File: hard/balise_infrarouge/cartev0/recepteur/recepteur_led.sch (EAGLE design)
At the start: 112 parts, among them IC2 7805DT, IC3 4051D, IC4 4051D, IC5 AT90CAN128A, J1 CAN, Q2 16M, X4 UART, X5 ISP

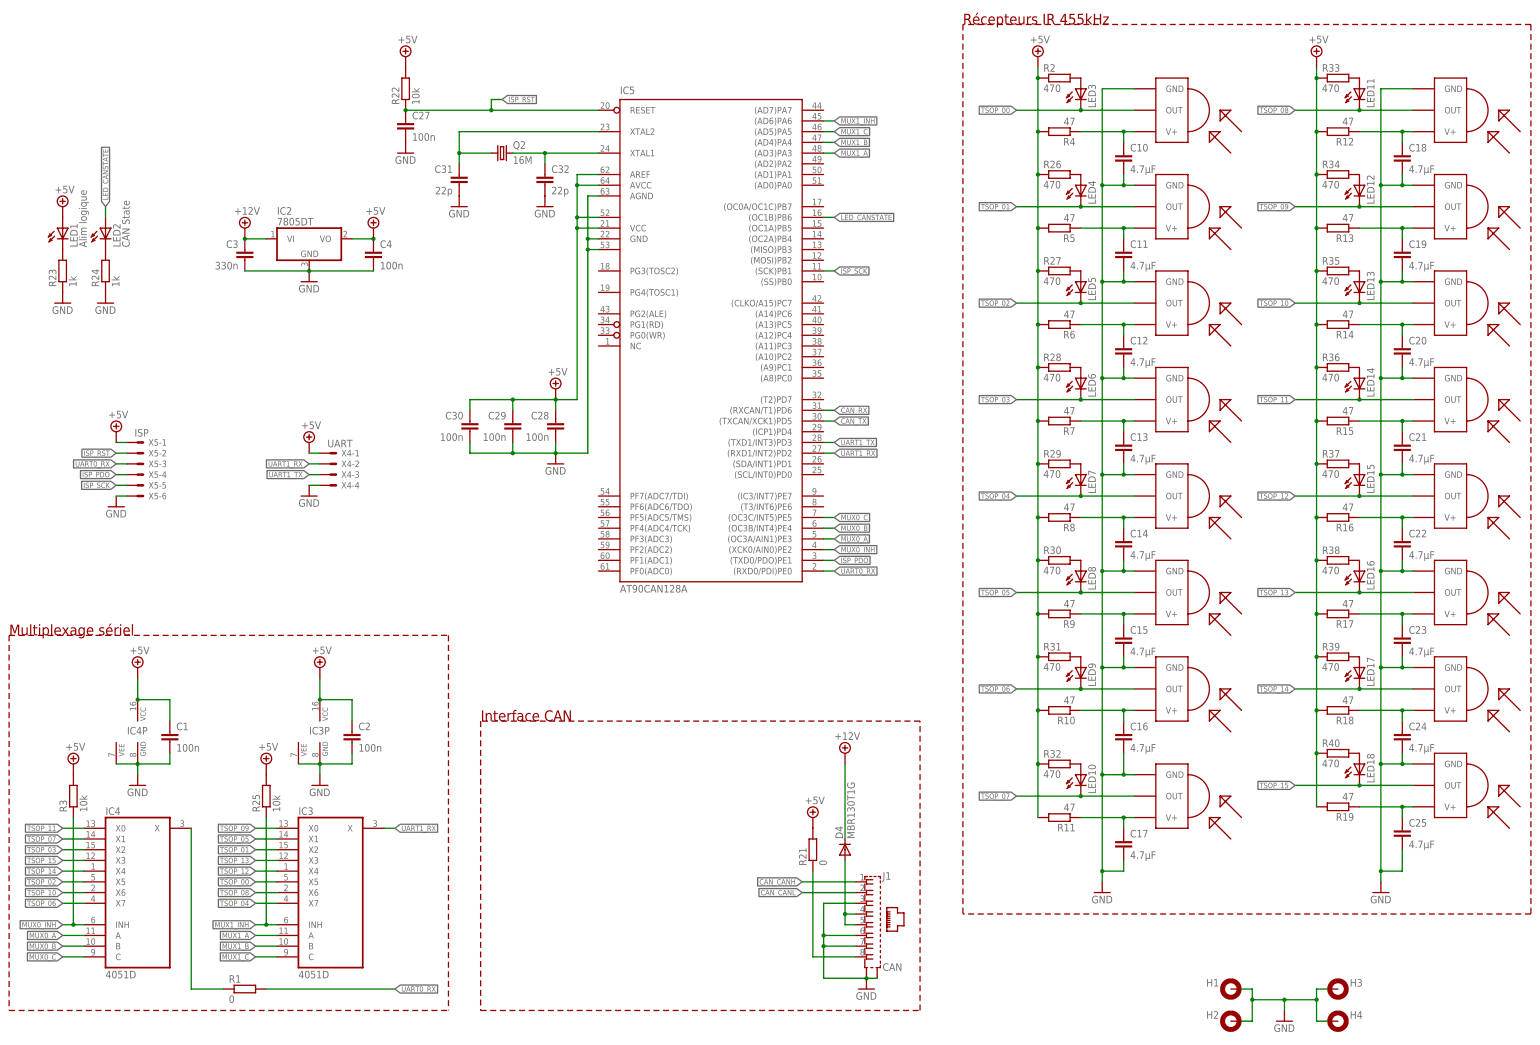
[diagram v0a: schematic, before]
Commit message: maj emetteur + fini recepteur part 1
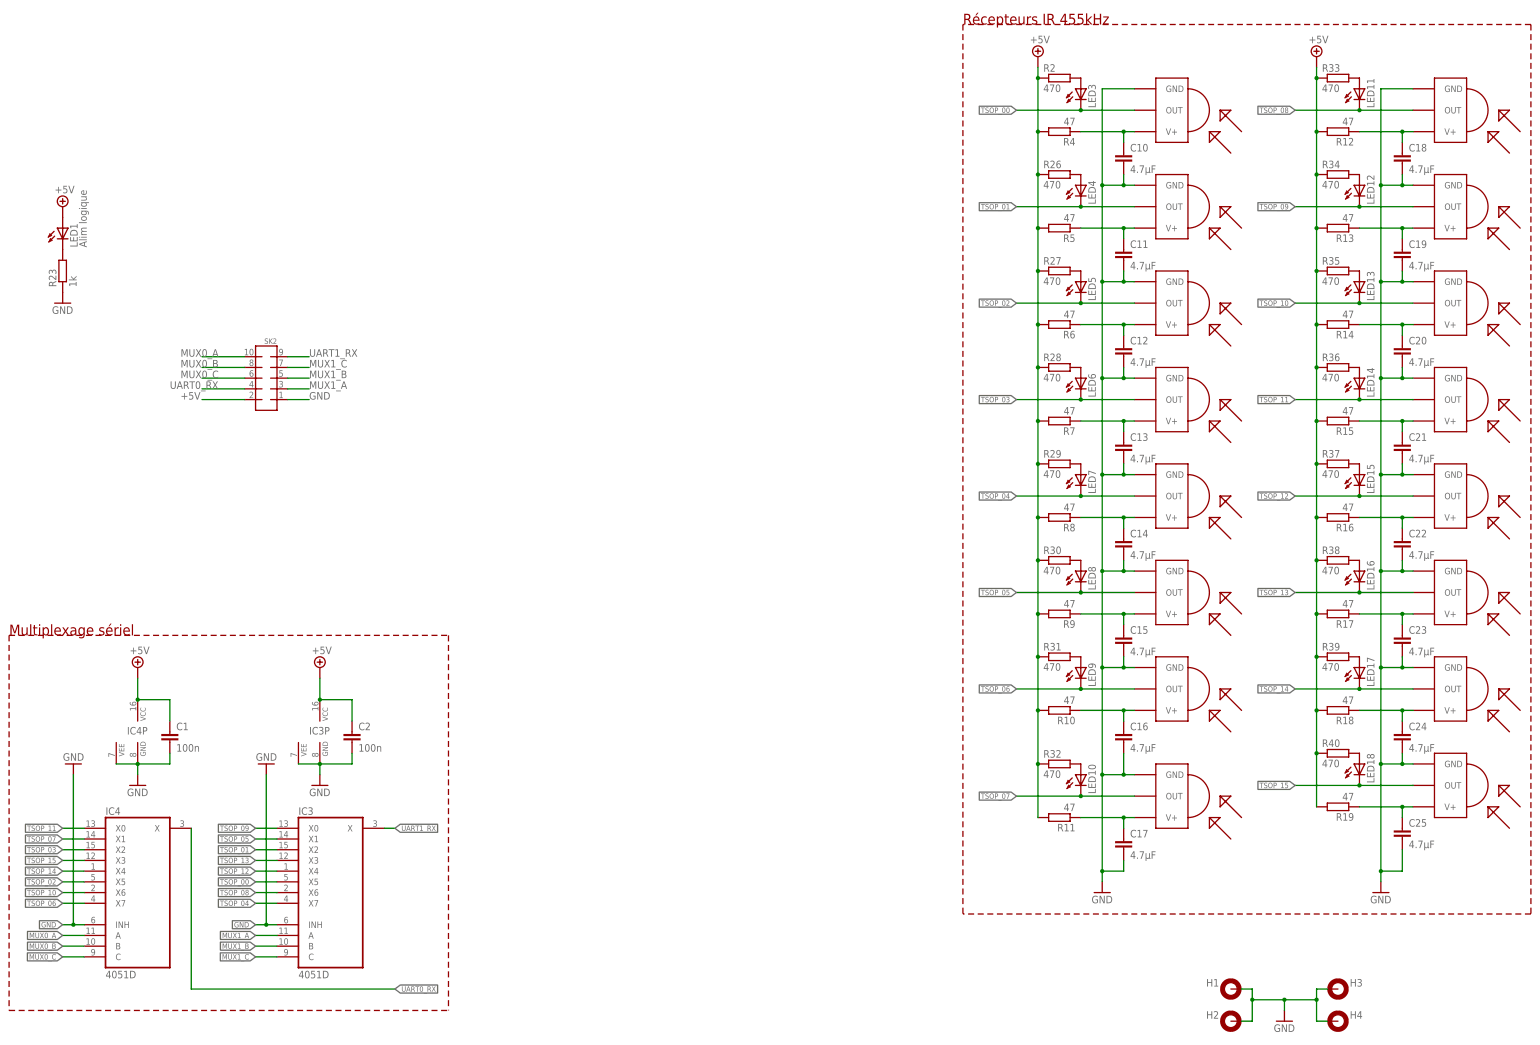
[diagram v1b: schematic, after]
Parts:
- removed C27, C28, C29, C30, C4: 100n, rcl:C-EUC0805
- removed C3: 330n, rcl:C-EUC0805
- removed C31, C32: 22p, rcl:C-EUC0805
- removed D4: MBR130T1G, diode:DIODE-SOD123
- removed IC2: 7805DT, linear:7805DT
- removed IC5: AT90CAN128A, avr:AT90CAN128A
- removed J1: CAN, con-amp:557969-1
- removed LED2: CAN State, led:LEDCHIP-LED0805
- removed Q2: 16M, crystal:CRYSTALHC49UP
- removed R1: 0, rcl:R-EU_R0805
- removed R21: 0, rcl:R-EU_M0805
- removed R22, R25, R3: 10k, rcl:R-EU_R0805
- removed R24: 1k, rcl:R-EU_M0805
- removed X4: UART, con-molex:53261-04
- removed X5: ISP, con-molex:53261-06
- added SK2: (no value), jt-con-micromatch:MMATCH-10-PTH
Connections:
- removed net +12V: C3.1, D4.C, IC2.VI
- removed net CAN_CANH: J1.1
- removed net CAN_CANL: J1.2
- removed net CAN_RX: IC5.(RXCAN/T1)PD6
- removed net CAN_TX: IC5.(TXCAN/XCK1)PD5
- removed net ISP_PDO: IC5.(TXD0/PDO)PE1, X5-4.S
- removed net ISP_RST: C27.1, IC5.RESET, R22.1, X5-2.S
- removed net ISP_SCK: IC5.(SCK)PB1, X5-5.S
- removed net LED_CANSTATE: IC5.(OC1B)PB6, LED2.A
- removed net MUX0_INH: IC4A.INH, IC5.(XCK0/AIN0)PE2, R3.1
- removed net MUX1_INH: IC3A.INH, IC5.(AD6)PA6, R25.1
- removed net N$1: IC4A.X, R1.1
- removed net N$13: C32.1, IC5.XTAL1, Q2.2
- removed net N$14: C31.1, IC5.XTAL2, Q2.1
- removed net N$17: LED2.C, R24.2
- removed net N$34: D4.A, J1.4, J1.5
- removed net N$8: J1.8, R21.1
- removed net UART1_TX: IC5.(TXD1/INT3)PD3, X4-3.S
- net +5V: now also SK2.2; no longer C28.1, C29.1, C30.1, C4.1, IC2.VO, IC5.AREF, IC5.AVCC, IC5.VCC, IC5.VCC1, R21.2, R22.2, R25.2, R3.2, X4-1.S, X5-1.S
- net GND: now also IC3A.INH, IC4A.INH, SK2.1; no longer C27.2, C28.2, C29.2, C3.2, C30.2, C31.2, C32.2, C4.2, IC2.GND, IC5.AGND, IC5.GND, IC5.GND1, J1.3, J1.6, J1.7, J1.S1, J1.S2, R24.1, X4-4.S, X5-6.S
- net MUX0_A: now also SK2.10; no longer IC5.(OC3A/AIN1)PE3
- net MUX0_B: now also SK2.8; no longer IC5.(OC3B/INT4)PE4
- net MUX0_C: now also SK2.6; no longer IC5.(OC3C/INT5)PE5
- net MUX1_A: now also SK2.3; no longer IC5.(AD3)PA3
- net MUX1_B: now also SK2.5; no longer IC5.(AD4)PA4
- net MUX1_C: now also SK2.7; no longer IC5.(AD5)PA5
- net UART0_RX: now also IC4A.X, SK2.4; no longer IC5.(RXD0/PDI)PE0, R1.2, X5-3.S
- net UART1_RX: now also SK2.9; no longer IC5.(RXD1/INT2)PD2, X4-2.S
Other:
- note removed: "Interface CAN"
